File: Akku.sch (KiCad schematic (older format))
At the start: 49 parts, among them J1 +/- Stecker, J2 load/up, J3 down/en/clear, P7 CONN_02X10, P8 CONN_02X10, P9 CONN_02X10, SW1 UP_Bonsai_SWITCH_INV, SW2 DOWN_Bonsai_SWITCH_INV, SW3 CLR_Bonsai_SWITCH_INV, U1 74HC14, U2 7400, U4 7408, U5 74LS193, U6 74LS541, U7 74LS193, U8 74LS540

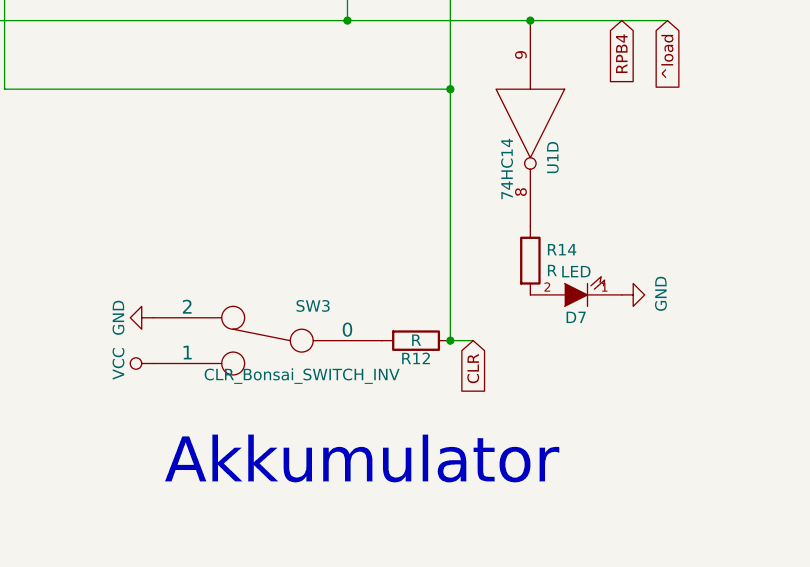
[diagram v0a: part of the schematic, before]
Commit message: akku and wireing in pcb
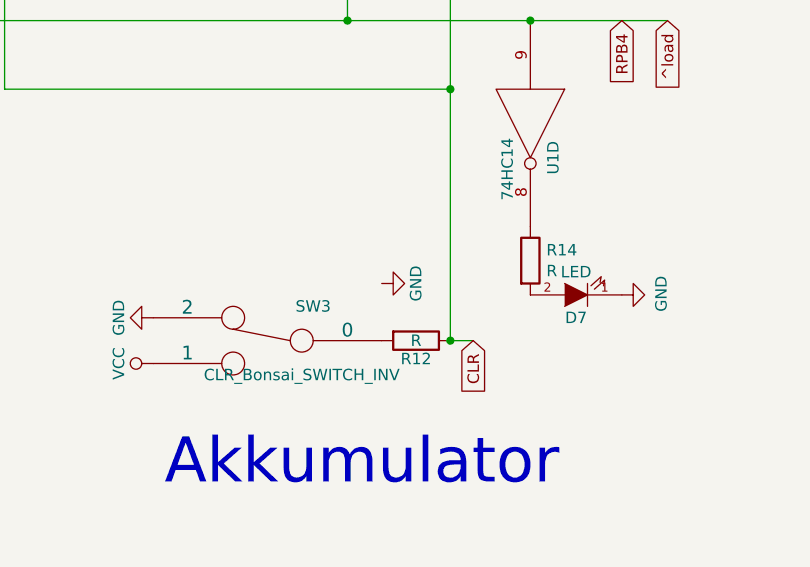
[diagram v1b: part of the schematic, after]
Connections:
- net GND: now also SW3.6
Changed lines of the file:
@@
 Connection ~ 850  1600
 Connection ~ 1150 1600
+$Comp
+L power:GND #PWR?
+U 1 1 5CDAAA47
+P 8000 5950
+F 0 "#PWR?" H 8000 5700 50  0001 C CNN
+F 1 "GND" H 8000 5800 50  0000 C CNN
+F 2 "" H 8000 5950 50  0000 C CNN
+F 3 "" H 8000 5950 50  0000 C CNN
+	1    8000 5950
+	0    -1   -1   0
+$EndComp
 Wire Bus Line
 	5250 600  5250 2100

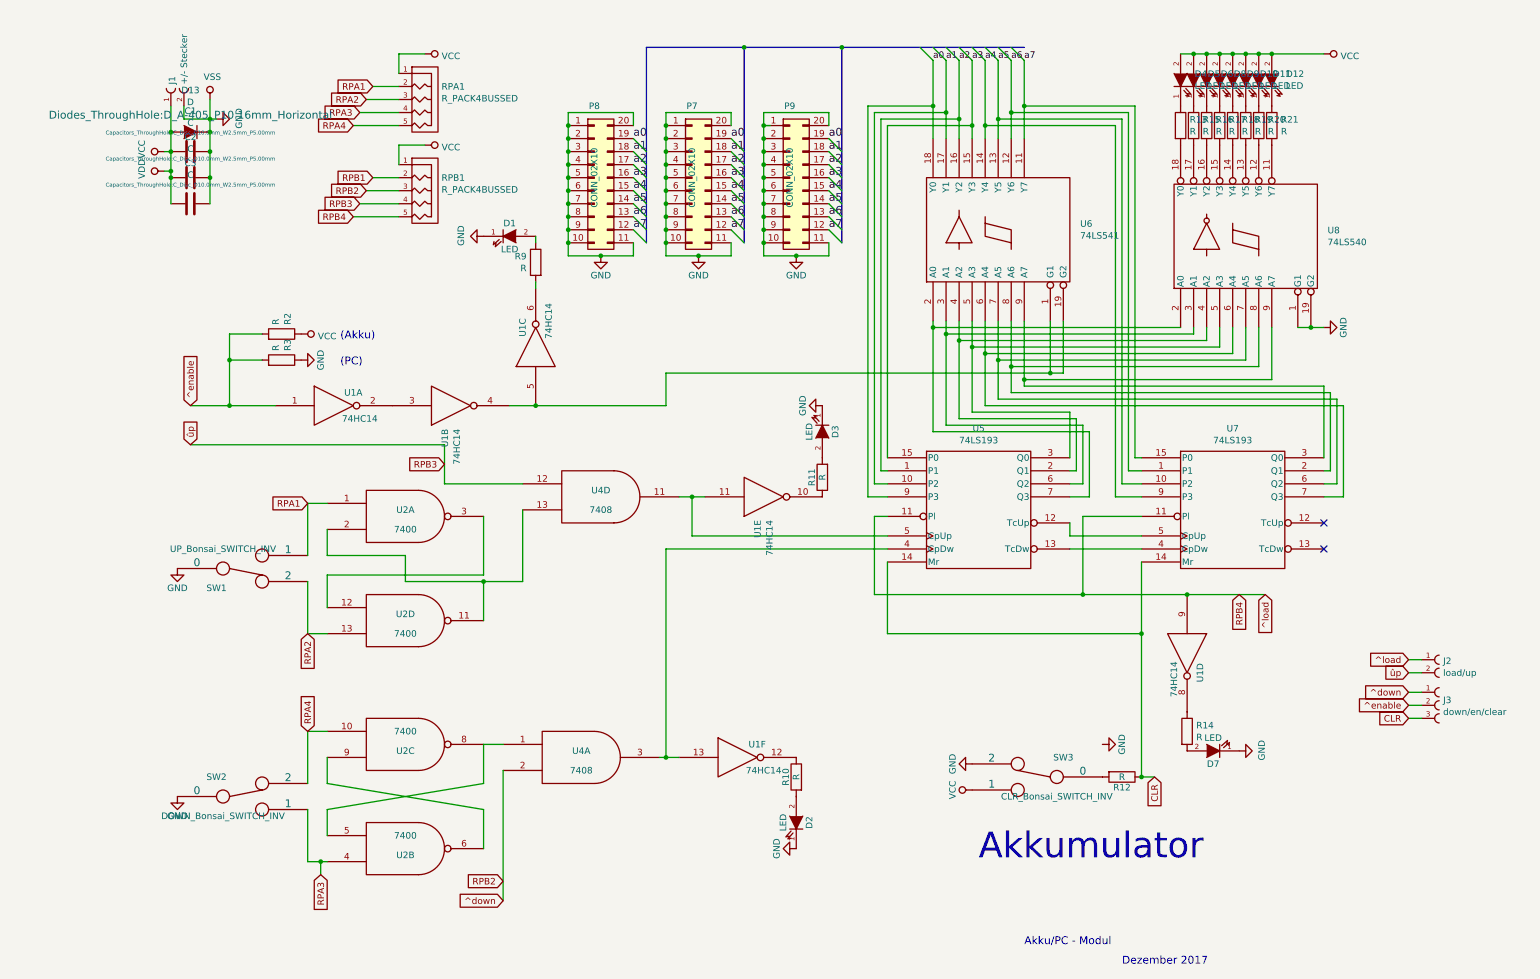
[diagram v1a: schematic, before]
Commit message: Akku pc finished
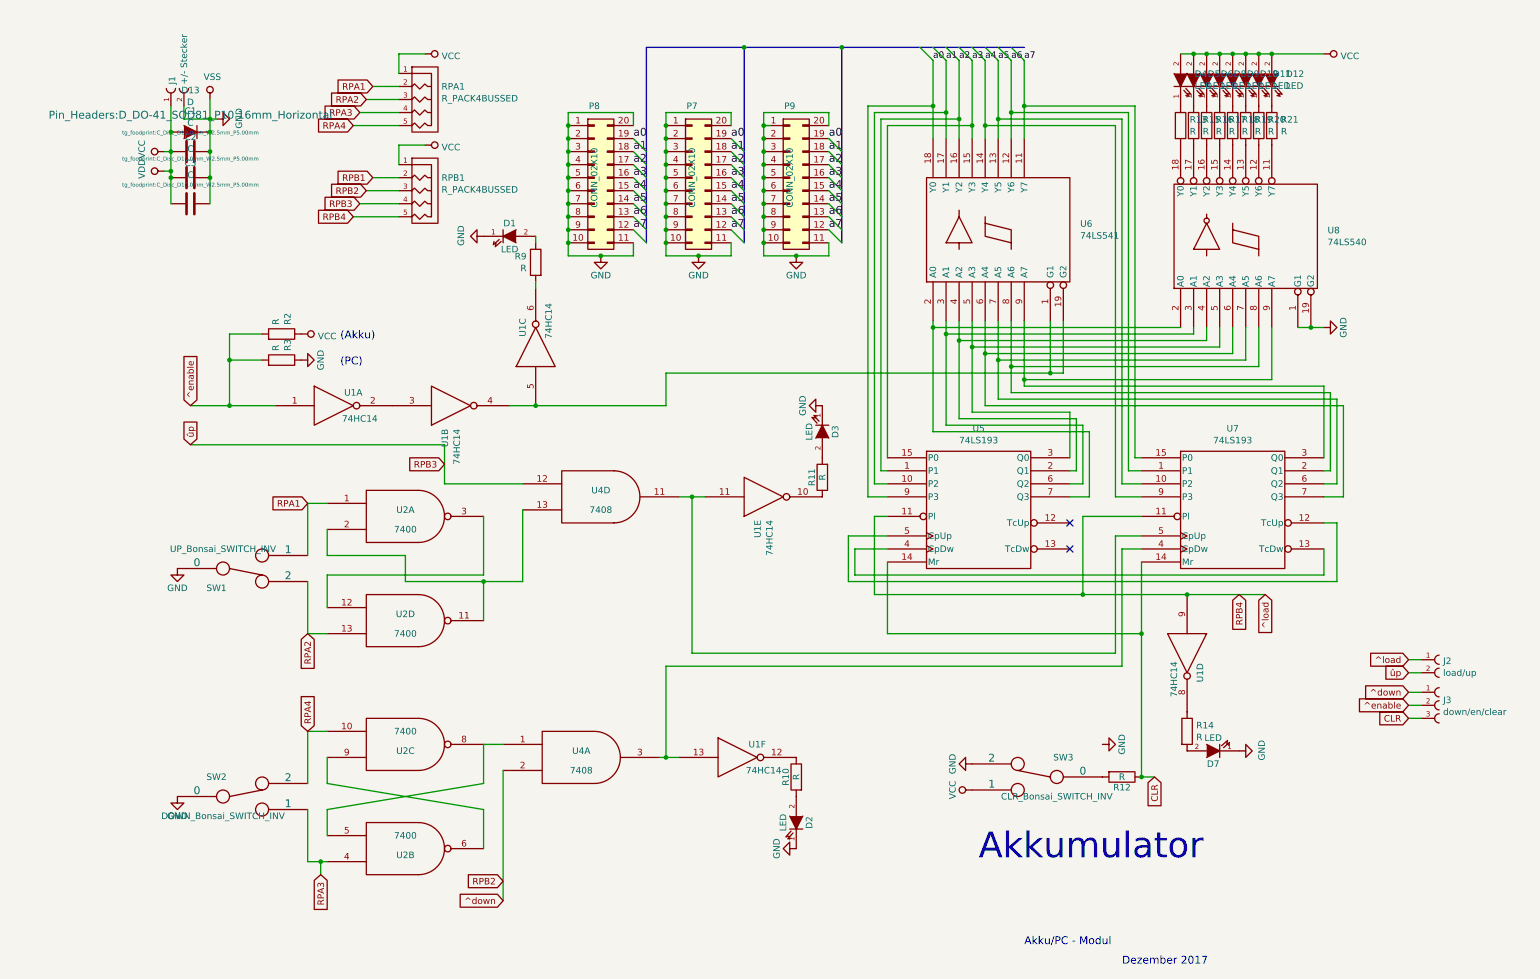
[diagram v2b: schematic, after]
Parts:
- C1, C2, C3: footprint Capacitors_ThroughHole:C_Disc_D10.0mm_W2.5mm_P5.00mm -> tg_foodprint:C_Disc_D10.0mm_W2.5mm_P5.00mm
- D13: footprint Diodes_ThroughHole:D_A-405_P10.16mm_Horizontal -> Pin_Headers:D_DO-41_SOD81_P10.16mm_Horizontal
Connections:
- net at U5.12 (TcUp): no longer U7.5 (CpUp)
- net at U5.13 (TcDw): no longer U7.4 (CpDw)
- net at U1.13, U4.3: now also U7.4 (CpDw); no longer U5.4 (CpDw)
- net at U1.11, U4.11: now also U7.5 (CpUp); no longer U5.5 (CpUp)
- net at U7.12 (TcUp): now also U5.5 (CpUp)
- net at U7.13 (TcDw): now also U5.4 (CpDw)
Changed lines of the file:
@@
 Wire Wire Line
 	8300 4550 8300 5100
-Wire Wire Line
-	4650 4450 6350 4450
 Connection ~ 4650 6050
-Wire Wire Line
-	4650 4450 4650 6050
 Wire Wire Line
 	4600 6050 4650 6050
@@
 	8300 5100 6350 5100
 Wire Wire Line
-	7750 4350 7750 4250
-Wire Wire Line
-	8300 4350 7750 4350
-Wire Wire Line
 	6250 4200 6350 4200
 Wire Wire Line
@@
 Wire Wire Line
 	7300 2700 7300 3050
-Wire Wire Line
-	7750 4450 8300 4450
-NoConn ~ 9700 4250
-NoConn ~ 9700 4450
 $Comp
 L Akku-rescue:74HC14-RESCUE-Akku U1
@@
 Connection ~ 9600 2750
 Wire Wire Line
-	6350 4350 4850 4350
-Wire Wire Line
-	4850 4350 4850 4050
+	6350 4350 6050 4350
 Connection ~ 4850 4050
 Wire Wire Line
@@
 F 0 "C1" V 688 1400 50  0000 C CNN
 F 1 "C" V 779 1400 50  0000 C CNN
-F 2 "Capacitors_ThroughHole:C_Disc_D10.0mm_W2.5mm_P5.00mm" V 855 1400 30  0000 C CNN
+F 2 "tg_foodprint:C_Disc_D10.0mm_W2.5mm_P5.00mm" V 855 1400 30  0000 C CNN
 F 3 "" H 1000 1400 60  0000 C CNN
 	1    1000 1400
@@
 F 0 "C2" V 688 1600 50  0000 C CNN
 F 1 "C" V 779 1600 50  0000 C CNN
-F 2 "Capacitors_ThroughHole:C_Disc_D10.0mm_W2.5mm_P5.00mm" V 855 1600 30  0000 C CNN
+F 2 "tg_foodprint:C_Disc_D10.0mm_W2.5mm_P5.00mm" V 855 1600 30  0000 C CNN
 F 3 "" H 1000 1600 60  0000 C CNN
 	1    1000 1600
@@
 F 0 "D13" H 1000 929 50  0000 C CNN
 F 1 "D" H 1000 1020 50  0000 C CNN
-F 2 "Diodes_ThroughHole:D_A-405_P10.16mm_Horizontal" H 1000 1119 60  0000 C CNN
+F 2 "Pin_Headers:D_DO-41_SOD81_P10.16mm_Horizontal" H 1000 1119 60  0000 C CNN
 F 3 "" H 1000 1250 60  0000 C CNN
 	1    1000 1250
@@
 F 0 "C3" V 688 1800 50  0000 C CNN
 F 1 "C" V 779 1800 50  0000 C CNN
-F 2 "Capacitors_ThroughHole:C_Disc_D10.0mm_W2.5mm_P5.00mm" V 855 1800 30  0000 C CNN
+F 2 "tg_foodprint:C_Disc_D10.0mm_W2.5mm_P5.00mm" V 855 1800 30  0000 C CNN
 F 3 "" H 1000 1800 60  0000 C CNN
 	1    1000 1800
@@
 Connection ~ 1150 1600
 $Comp
-L power:GND #PWR?
+L power:GND #PWR0104
 U 1 1 5CDAAA47
 P 8000 5950
-F 0 "#PWR?" H 8000 5700 50  0001 C CNN
+F 0 "#PWR0104" H 8000 5700 50  0001 C CNN
 F 1 "GND" H 8000 5800 50  0000 C CNN
 F 2 "" H 8000 5950 50  0000 C CNN
@@
 	0    -1   -1   0
 $EndComp
+Wire Wire Line
+	9700 4450 9700 4650
+Wire Wire Line
+	9700 4650 6100 4650
+Wire Wire Line
+	6100 4650 6100 4450
+Wire Wire Line
+	9700 4250 9800 4250
+Wire Wire Line
+	9800 4250 9800 4700
+Wire Wire Line
+	8300 4450 8150 4450
+Wire Wire Line
+	8150 4450 8150 5350
+Wire Wire Line
+	8150 5350 4650 5350
+Wire Wire Line
+	4650 5350 4650 6050
+Wire Wire Line
+	6050 4700 6050 4350
+Wire Wire Line
+	9800 4700 6050 4700
+Wire Wire Line
+	8300 4350 8100 4350
+Wire Wire Line
+	8100 4350 8100 5250
+Wire Wire Line
+	8100 5250 4850 5250
+Wire Wire Line
+	4850 4050 4850 5250
+NoConn ~ 7750 4250
+NoConn ~ 7750 4450
+Wire Wire Line
+	6350 4450 6100 4450
+Wire Bus Line
+	6000 600  7400 600
+Wire Bus Line
+	4500 600  4500 2100
 Wire Bus Line
 	5250 600  5250 2100
 Wire Bus Line
-	4500 600  4500 2100
-Wire Bus Line
 	6000 600  6000 2100
-Wire Bus Line
-	6000 600  7400 600
 $EndSCHEMATC
